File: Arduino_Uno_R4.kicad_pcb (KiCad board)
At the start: 2 copper layers, 48.9 x 38.1 mm, 55 parts, among them J1 Jack-DC, J17 ICSP1, J2 ICSP2, J3 USB_B, J4 PORTB, J5 PWR_PORT, J6 PORTC, J7 PORTD, Q1 FDN340P, SW1 RES, U1 LMV358, U2 LP2985-3.3, U3 NCP1117ST50, U5 ATmega16U2-MU, U6 ATmega328P-MU, Y1 16MHz, Y2 16MHz

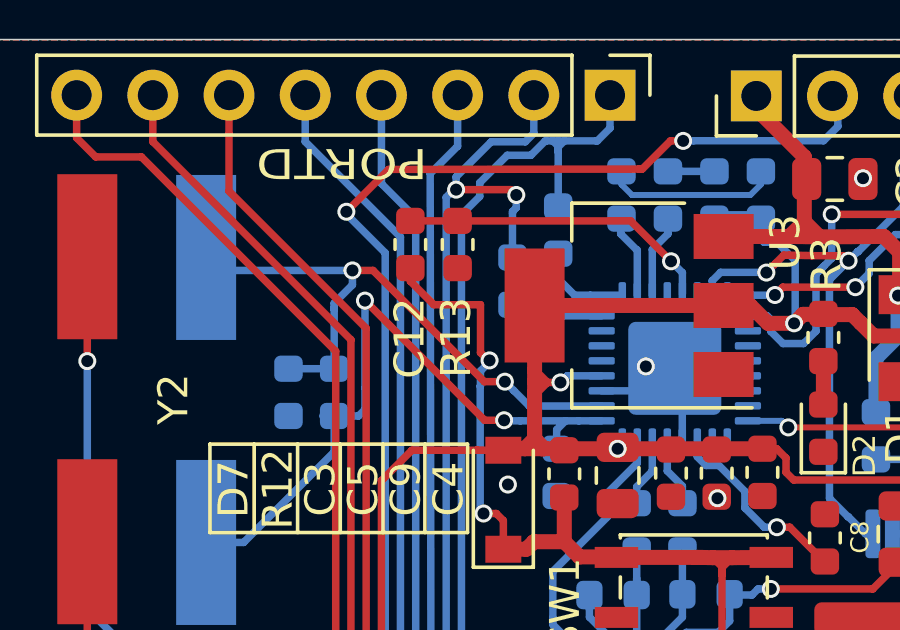
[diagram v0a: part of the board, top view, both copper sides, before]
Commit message: Generated GERBER and drill files
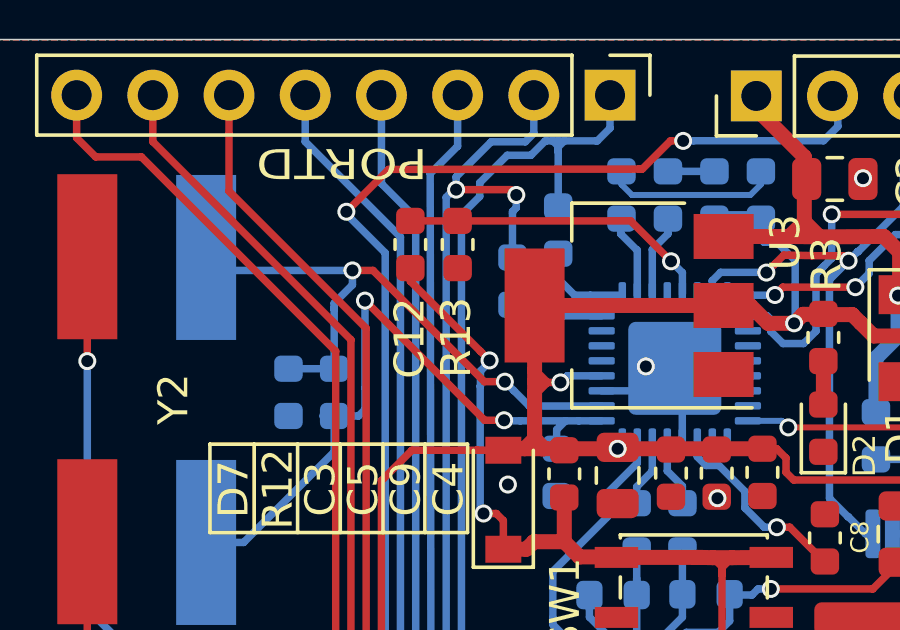
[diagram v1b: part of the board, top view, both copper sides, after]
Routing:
- net Net-(C12-Pad2): track 60.4 -> 59.4 mm
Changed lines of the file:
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@@
     (thickness 1.6)
     (drawings 24)
-    (tracks 860)
+    (tracks 858)
     (zones 0)
     (modules 55)
@@
     (0 F.Cu signal)
     (31 B.Cu signal)
-    (34 B.Paste user)
-    (35 F.Paste user)
     (36 B.SilkS user)
     (37 F.SilkS user)
     (38 B.Mask user)
     (39 F.Mask user)
-    (40 Dwgs.User user)
+    (40 Dwgs.User user hide)
     (44 Edge.Cuts user)
-    (45 Margin user)
-    (46 B.CrtYd user)
-    (47 F.CrtYd user)
-    (48 B.Fab user)
-    (49 F.Fab user)
+    (45 Margin user hide)
+    (46 B.CrtYd user hide)
+    (47 F.CrtYd user hide)
+    (48 B.Fab user hide)
+    (49 F.Fab user hide)
   )
   (setup
@@
     (visible_elements 7FFFFFFF)
     (pcbplotparams
-      (layerselection 0x010fc_ffffffff)
+      (layerselection 0x010f0_ffffffff)
       (usegerberextensions false)
       (usegerberattributes false)
@@
       (outputformat 1)
       (mirror false)
-      (drillshape 1)
+      (drillshape 0)
       (scaleselection 1)
       (outputdirectory ""))
@@
   (segment (start 72.009 75.7174) (end 72.644 75.7174) (width 0.5) (layer F.Cu) (net 8))
   (segment (start 72.644 75.7174) (end 73.898 75.708) (width 0.5) (layer F.Cu) (net 8))
-  (segment (start 63.837736 67.2846) (end 64.262 67.2846) (width 0.25) (layer F.Cu) (net 8))
-  (segment (start 62.7069 67.2846) (end 63.837736 67.2846) (width 0.25) (layer F.Cu) (net 8))
-  (segment (start 61.9252 66.5029) (end 62.7069 67.2846) (width 0.25) (layer F.Cu) (net 8))
-  (segment (start 61.9252 66.0654) (end 61.9252 66.5029) (width 0.25) (layer F.Cu) (net 8))
   (segment (start 64.252 70.0024) (end 64.262 69.9924) (width 0.25) (layer B.Cu) (net 8))
   (via (at 64.564242 69.141358) (size 0.6) (drill 0.4) (layers F.Cu B.Cu) (net 8))
-  (segment (start 64.262 67.2846) (end 64.262 68.8848) (width 0.25) (layer F.Cu) (net 8))
-  (segment (start 64.262 68.8848) (end 64.5668 69.1896) (width 0.25) (layer F.Cu) (net 8))
   (segment (start 64.262 69.4944) (end 64.262 69.9924) (width 0.25) (layer B.Cu) (net 8))
   (segment (start 64.5668 69.1896) (end 64.262 69.4944) (width 0.25) (layer B.Cu) (net 8))
+  (segment (start 61.9252 66.5029) (end 61.9252 66.0654) (width 0.25) (layer F.Cu) (net 8))
+  (segment (start 64.262 68.8397) (end 61.9252 66.5029) (width 0.25) (layer F.Cu) (net 8))
+  (segment (start 64.262584 68.8397) (end 64.262 68.8397) (width 0.25) (layer F.Cu) (net 8))
+  (segment (start 64.564242 69.141358) (end 64.262584 68.8397) (width 0.25) (layer F.Cu) (net 8))
   (segment (start 75.692 69.1642) (end 75.692 70.5866) (width 0.5) (layer F.Cu) (net 9))
   (segment (start 82.4992 73.9648) (end 84.1248 73.9648) (width 0.25) (layer B.Cu) (net 10))
